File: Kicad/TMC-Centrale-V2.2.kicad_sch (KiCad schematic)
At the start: 4 parts

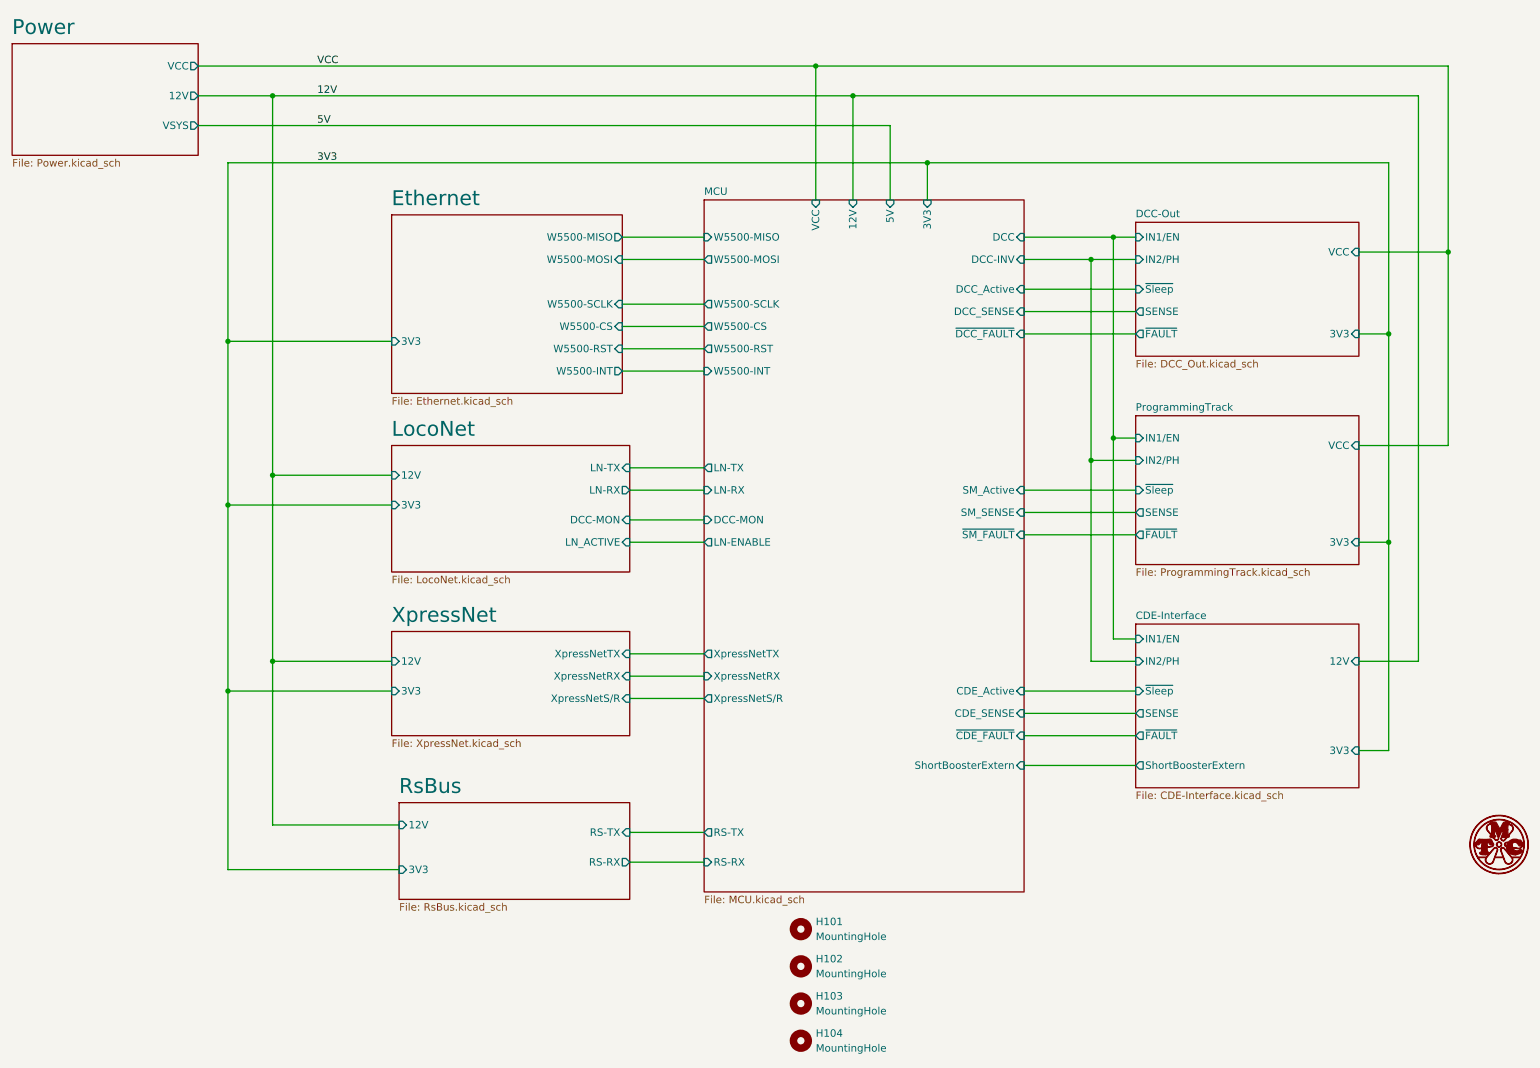
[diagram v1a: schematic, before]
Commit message: Centrale V2.3 (1)
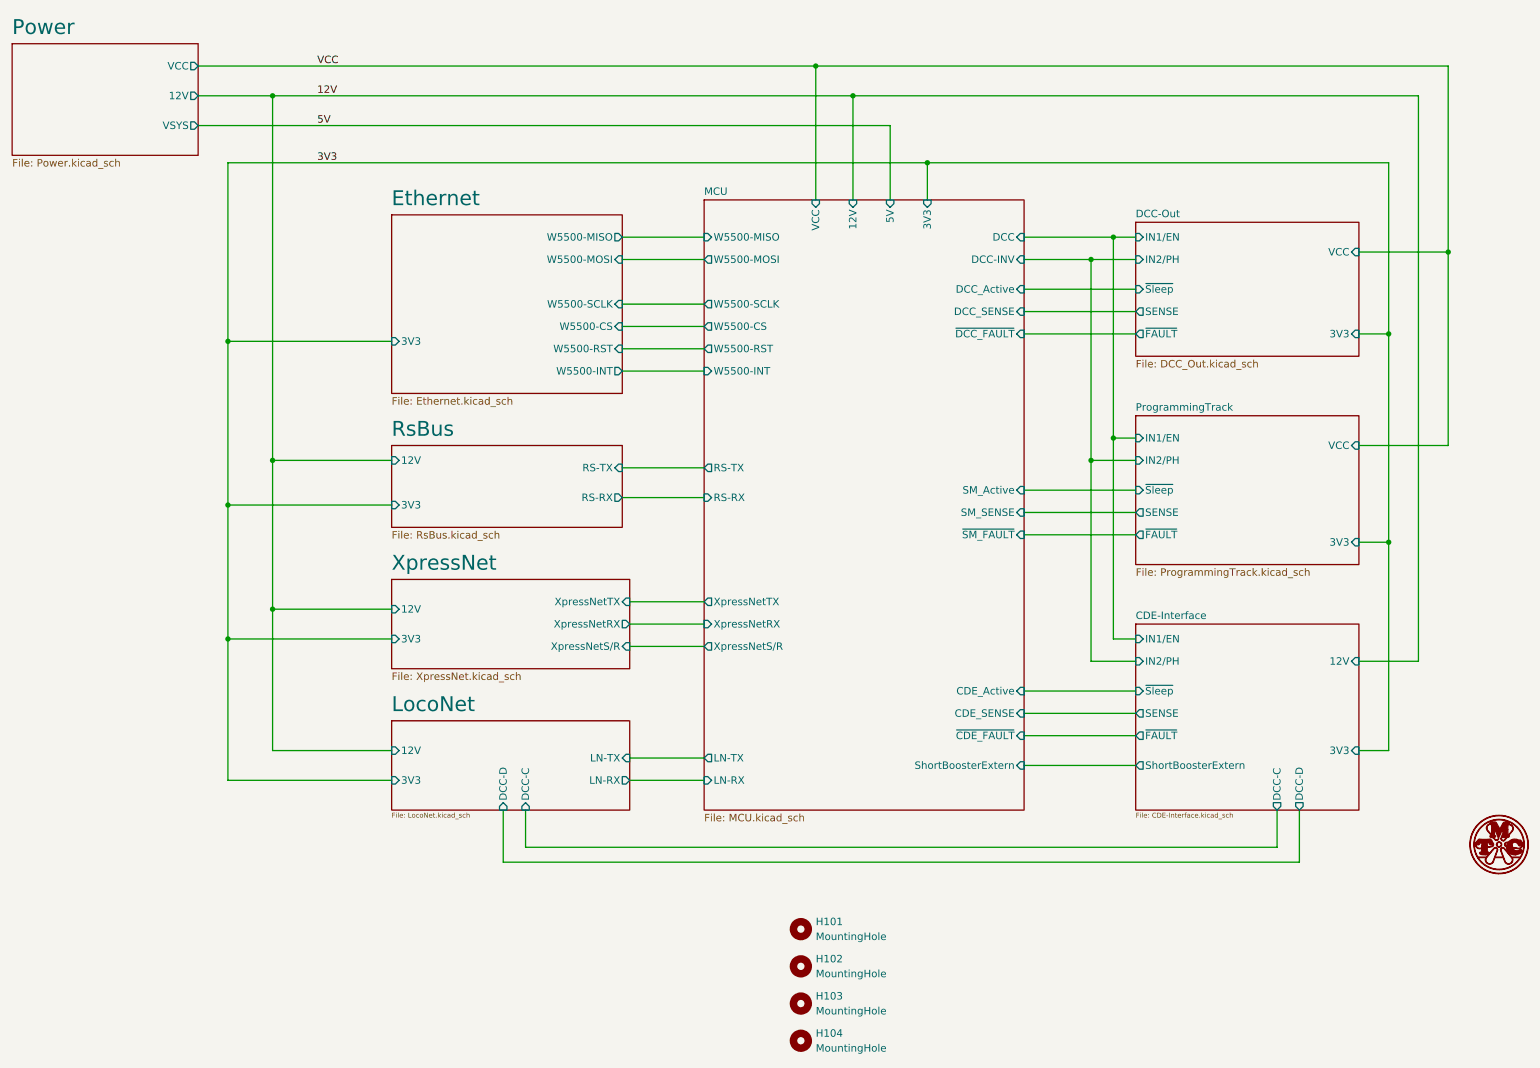
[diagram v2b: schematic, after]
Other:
- sheet CDE-Interface ports: added DCC-C, DCC-D; removed none
- sheet LocoNet ports: added DCC-C, DCC-D; removed DCC-MON, LN_ACTIVE
- sheet MCU ports: added none; removed DCC-MON, LN-ENABLE
